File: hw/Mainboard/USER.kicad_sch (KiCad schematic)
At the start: 3 parts, among them J26 USER_HEADER, J4 USER

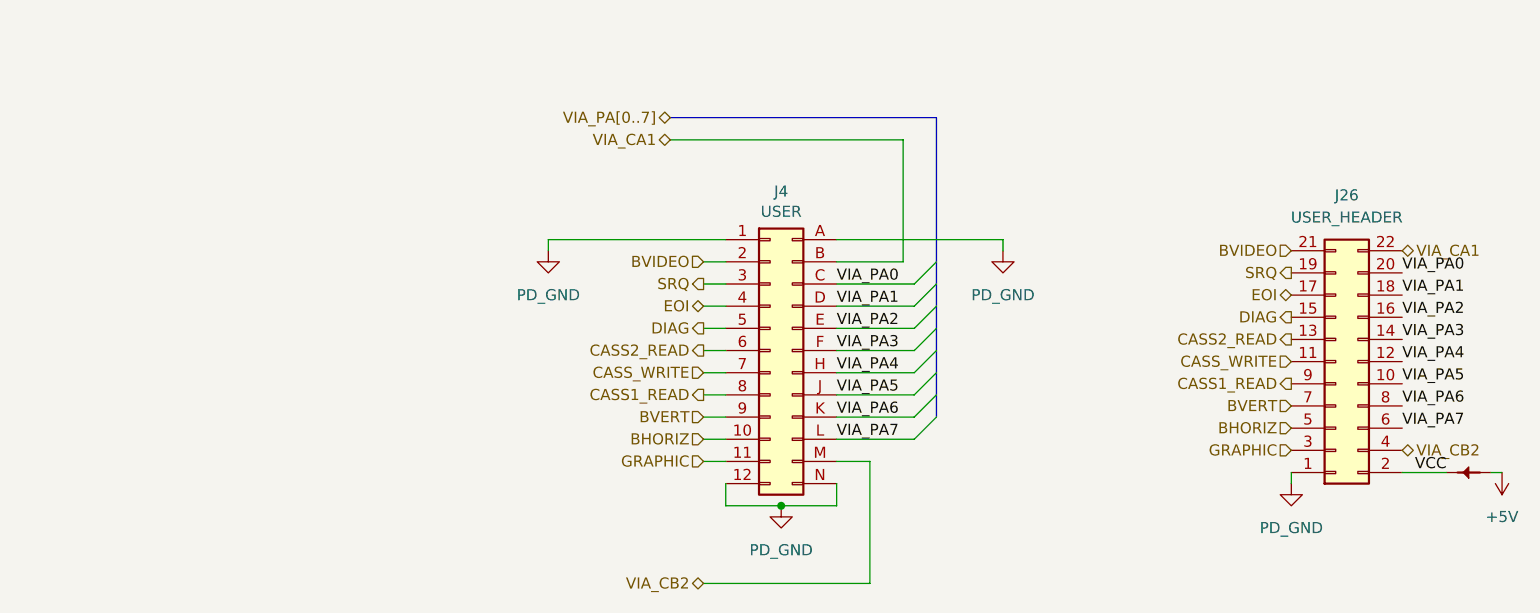
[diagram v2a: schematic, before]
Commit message: wip
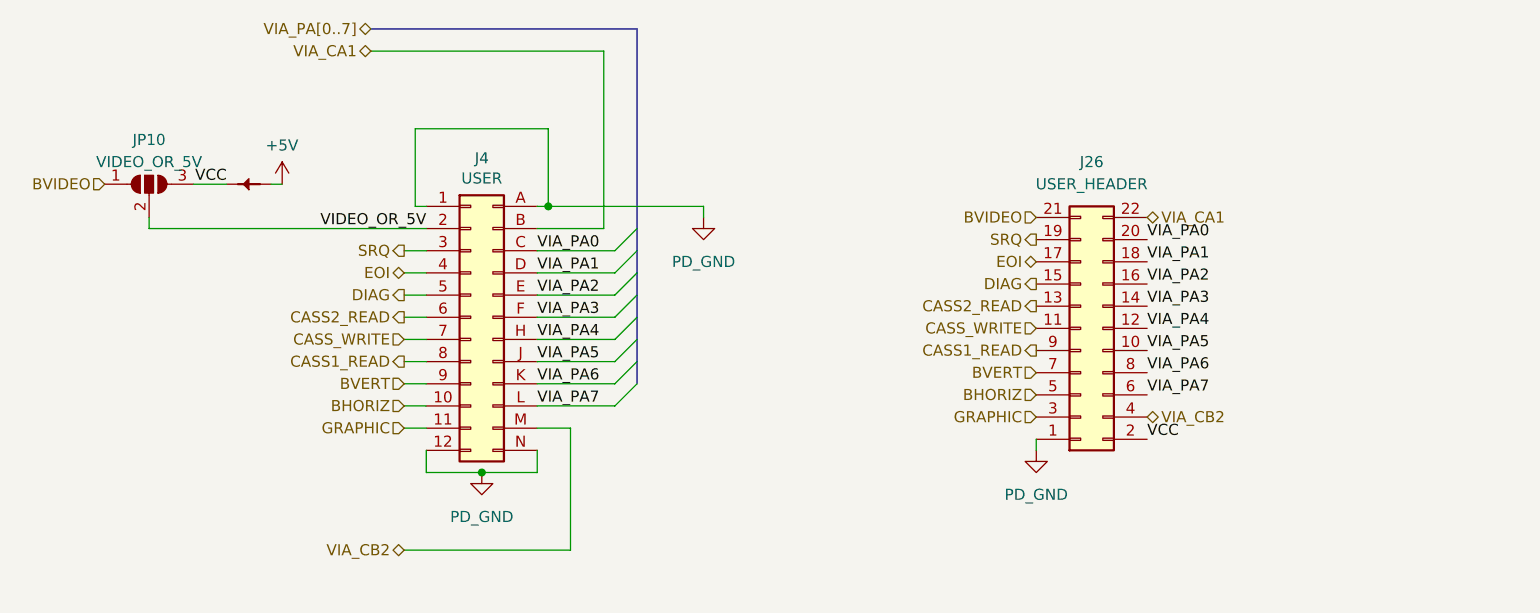
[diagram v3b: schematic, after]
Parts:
- added JP10: VIDEO_OR_5V, Jumper:SolderJumper-3_P1.3mm_Open_RoundedPad1.0x1.5mm, symbol Jumper:SolderJumper_3_Open
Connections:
- net BVIDEO: now also JP10.1 (A); no longer J4.2 (~{VIDEO})
- net VCC: now also JP10.3 (B)
- new net VIDEO_OR_5V: J4.2 (~{VIDEO}), JP10.2 (C)
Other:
- moved on the sheet: J26, J4
